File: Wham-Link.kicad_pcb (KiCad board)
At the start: 4 copper layers, 70 x 30 mm, 62 parts, among them J2 Conn_02x05_Counter_Clockwise, J3 Conn_01x09_Pin, Q1 2SC4617R, Q3 UMH3N, SW2 SKRPACE010, SW3 SKRPACE010, U1 LAN8720A-CP-TR, U2 AMS1117-3.3, U3 CH340C, U4 ESP32-WROOM-32UE, X1 ECS-2520MV-250-CN-TR

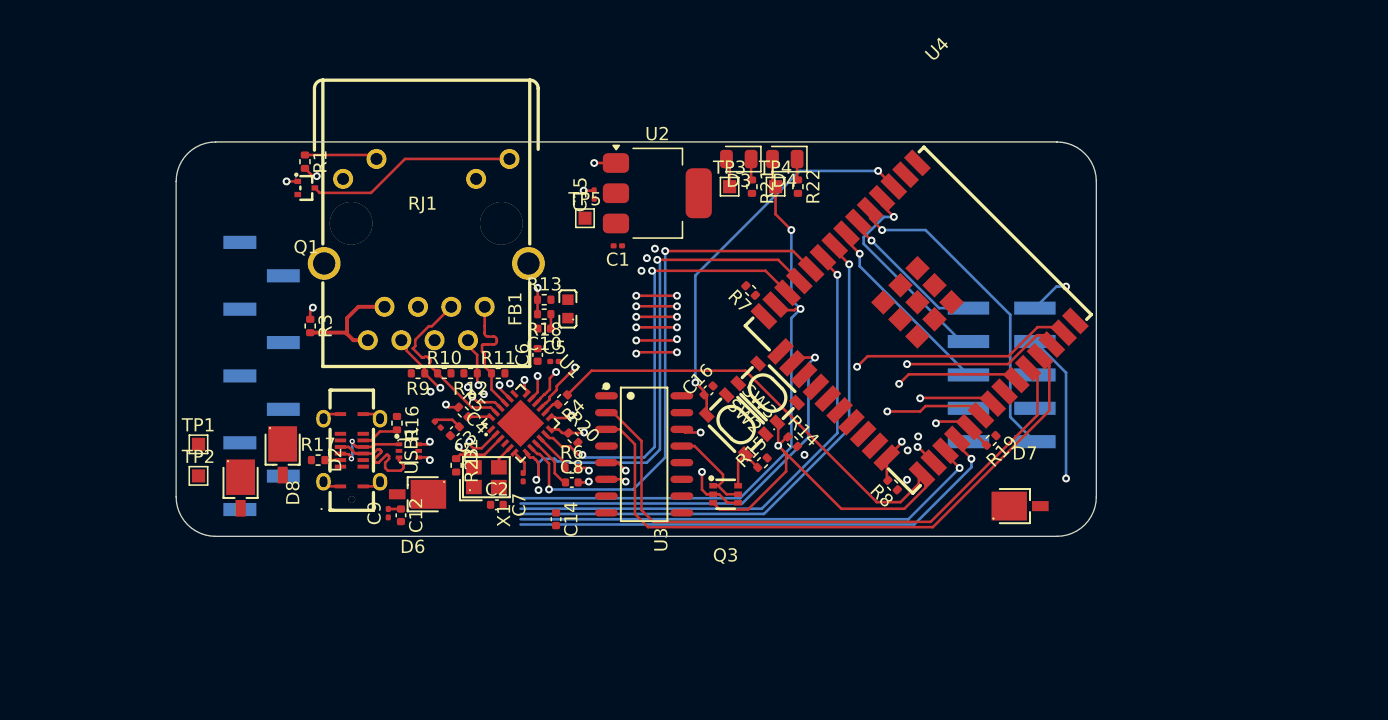
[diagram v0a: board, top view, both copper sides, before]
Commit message: re-layout
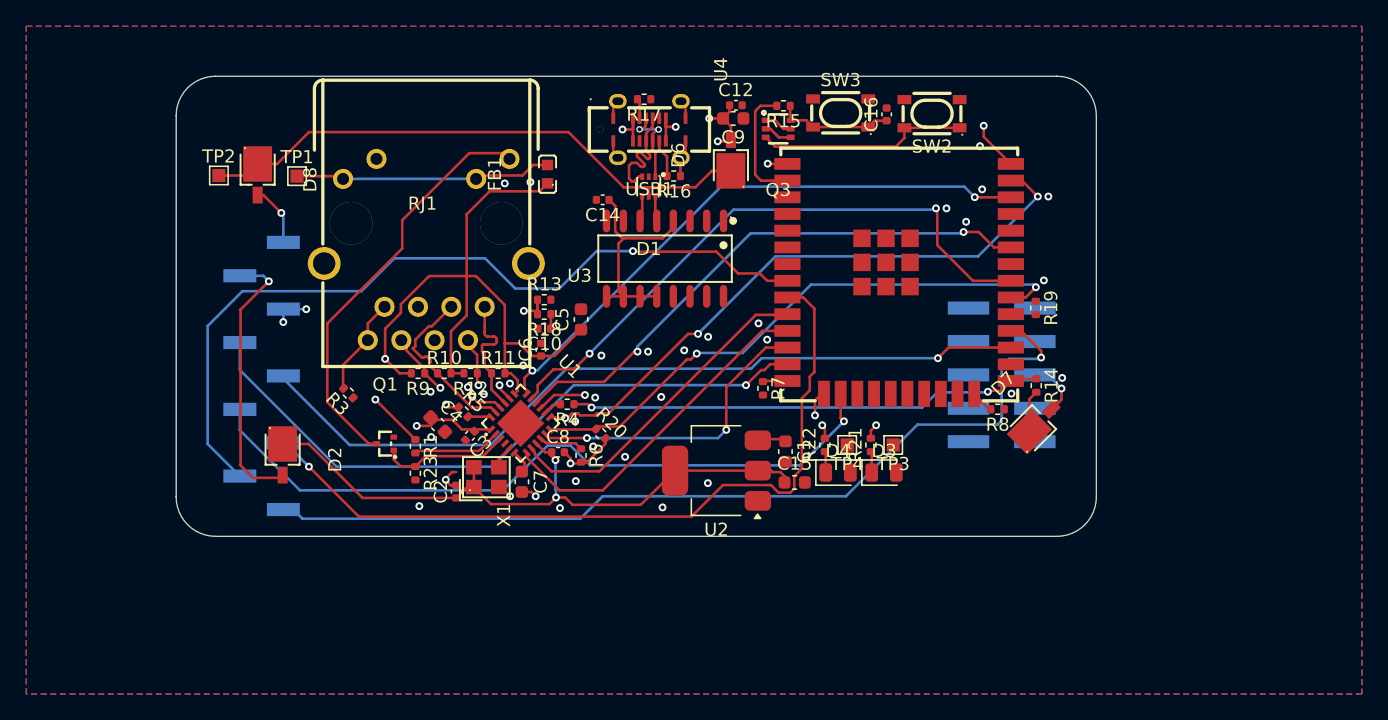
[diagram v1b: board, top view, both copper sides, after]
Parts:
- removed TP5: TestPoint_Small, TestPoint:TestPoint_Pad_1.0x1.0mm
- C1, C15, C4, C5, C7, C9: footprint Capacitor_SMD:C_0201_0603Metric -> Capacitor_SMD:C_0603_1608Metric
- moved C12 40.3 mm to (155.6, 82.2), turned to 0 degrees
- moved C9 39.9 mm to (155.4, 83.2), turned to 180 degrees
- moved R17 37.0 mm to (148.6, 81.8), turned to 180 degrees
- moved D6 35.4 mm to (155.2, 86.0), turned to 90 degrees
- moved USB1 33.3 mm to (149.0, 84.1), turned to 0 degrees
- moved R16 28.2 mm to (150.9, 87.6), turned to 180 degrees
- moved Q3 28.1 mm to (158.8, 84.0)
- moved R15 27.2 mm to (159.2, 82.2), turned to 180 degrees
- moved D1 27.2 mm to (149.0, 88.4), turned to 180 degrees
- moved C15 26.7 mm to (160.1, 110.9), turned to 0 degrees
- moved D3 26.3 mm to (166.8, 110.2), turned to 0 degrees
- moved SW3 25.0 mm to (163.6, 82.8), turned to 180 degrees
- moved C16 25.0 mm to (167.1, 82.9), turned to 90 degrees
- moved SW2 24.7 mm to (170.5, 82.8), turned to 180 degrees
- moved C14 24.6 mm to (145.4, 89.4), turned to 180 degrees
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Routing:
- net +3V3: track 6.18 -> 81.6 mm, vias 0 -> 2
- net /VDD1A: track 2.14 -> 64.3 mm, vias 0 -> 2
- net TXD0: track 48.0 -> 0.00 mm
- net RXD0: track 46.5 -> 0.00 mm
- net +5V: track 0.00 -> 45.9 mm
- net IO5: track 40.6 -> 3.78 mm, vias 4 -> 1
- net GP17: track 38.7 -> 68.9 mm
- net /LED2: track 34.7 -> 6.72 mm, vias 2 -> 0
- net /LED1: track 35.6 -> 9.92 mm, vias 2 -> 0
- net EN: track 33.9 -> 8.83 mm, vias 2 -> 0
- net GPI39: track 24.7 -> 0.00 mm, vias 1 -> 0
- net GP16: track 36.8 -> 60.7 mm
- net GP13: track 32.2 -> 55.0 mm
- net Net-(D2-A): track 0.00 -> 20.9 mm, vias 0 -> 1
- net GP32: track 42.1 -> 61.7 mm
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- added copper zone on B.Cu, net GND
- added copper zone on F.Cu, net GND
- added copper zone on In2.Cu, net Net-(D6-A)
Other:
- board size 70 x 30 mm -> 70 x 35 mm
